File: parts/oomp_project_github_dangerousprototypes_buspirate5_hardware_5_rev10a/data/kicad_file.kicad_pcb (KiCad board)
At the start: 4 copper layers, 80 x 80.2 mm, 220 parts, among them J201 Conn_01x03, J202 TYPE-C-31-M-12, J301 Conn_01x10, J302 Conn_01x09, Q202 MMBT7002K, Q300 SI2301, Q301 SI2301, Q302 SI2301, Q303 SI2301, Q304 SI2301, Q305 SI2301, Q306 SI2301, Q307 SI2301, Q401 BCM857, Q402 SI2301, Q601 MMDT3906, Q602 SI2301, SW101 SW_SPST, SW102 4P_button_sw, U102 W25Q128JVSIQ, U103 RP2040, U105 MT29F1G01ABAFDWB, U301 AiP74LVC1T45GC363.TR, U302 AiP74LVC1T45GC363.TR, U303 AiP74LVC1T45GC363.TR, U304 AiP74LVC1T45GC363.TR, U305 AiP74LVC1T45GC363.TR, U306 AiP74LVC1T45GC363.TR, U307 AiP74LVC1T45GC363.TR, U308 AiP74LVC1T45GC363.TR, U401 ME6211A33PG-N, U402 CD4067, U403 AP2127, U404 LMV321, U501 AIP74HC595TA, U502 AIP74HC595TA, U503 AIP74HCT245TA, U504 LMV324, U505 LMV324, U506 LMV321, U601 LMV321A, U602 LMV331, U603 LMV321, Y101 12Mhz

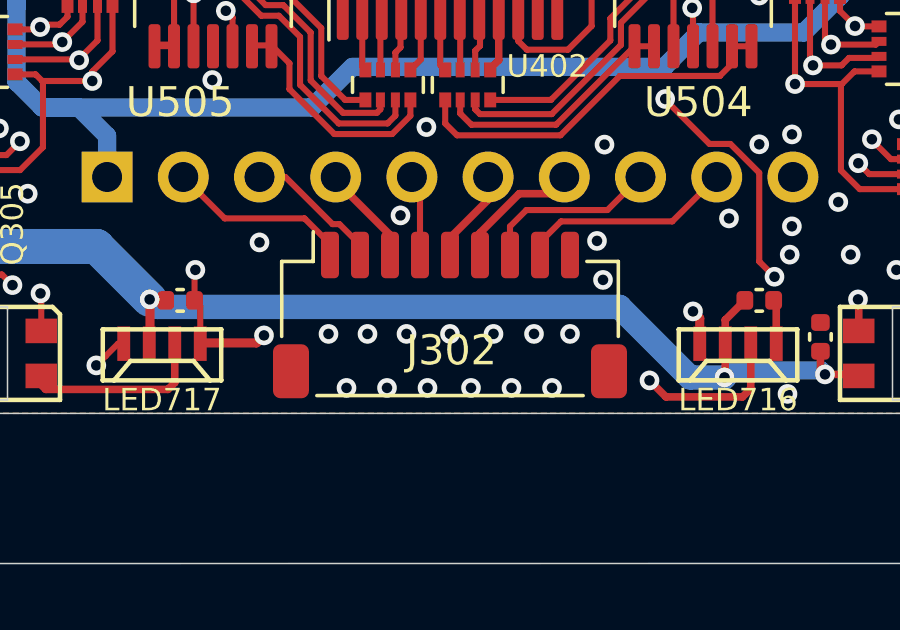
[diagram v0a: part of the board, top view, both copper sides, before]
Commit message: changes
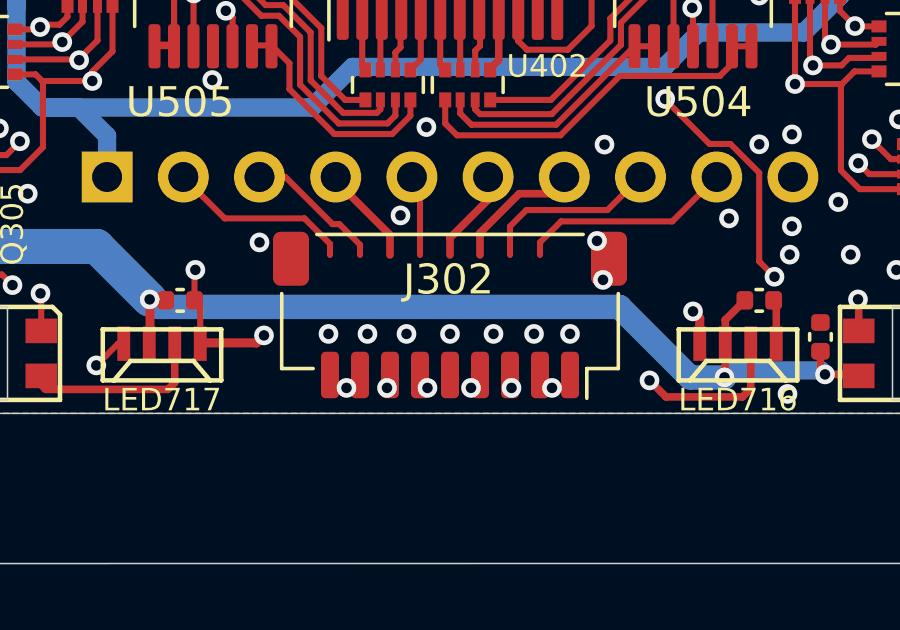
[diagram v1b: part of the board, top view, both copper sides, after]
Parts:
- turned J302 to 180 degrees
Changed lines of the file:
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@@
   )
   (footprint "Connector_JST:JST_SH_SM09B-SRSS-TB_1x09-1MP_P1.00mm_Horizontal" (layer "F.Cu")
-    (at 129.9 116.82)
+    (at 129.9 116.82 180)
     (descr "JST SH series connector, SM09B-SRSS-TB (http://www.jst-mfg.com/product/pdf/eng/eSH.pdf), generated with kicad-footprint-generator")
     (tags "connector JST SH top entry")

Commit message: major
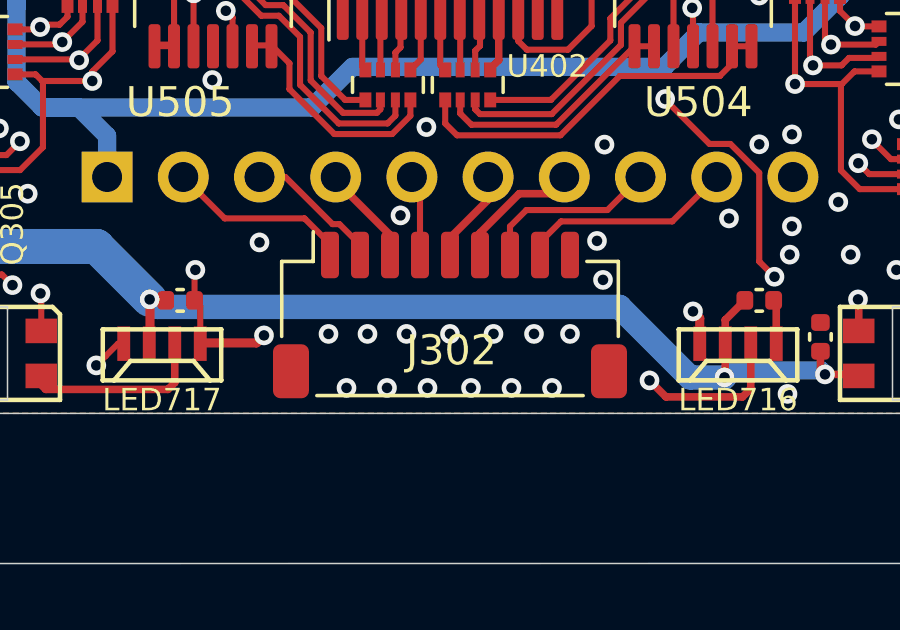
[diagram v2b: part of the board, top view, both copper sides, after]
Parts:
- turned J302 to 0 degrees
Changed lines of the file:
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@@
   )
   (footprint "Connector_JST:JST_SH_SM09B-SRSS-TB_1x09-1MP_P1.00mm_Horizontal" (layer "F.Cu")
-    (at 129.9 116.82 180)
+    (at 129.9 116.82)
     (descr "JST SH series connector, SM09B-SRSS-TB (http://www.jst-mfg.com/product/pdf/eng/eSH.pdf), generated with kicad-footprint-generator")
     (tags "connector JST SH top entry")
